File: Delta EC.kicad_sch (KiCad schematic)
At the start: 43 parts, among them J1 USB_C_Receptacle_USB2.0_16P, J2 SOICbite, J3 FFC Daughter side, J4 FFC Main side, J5 JSB USB, U1 STM32G474CBTx, U2 USBLC6-2SC6, U3 TPS7A2033, Y1 8Mhz 12pF

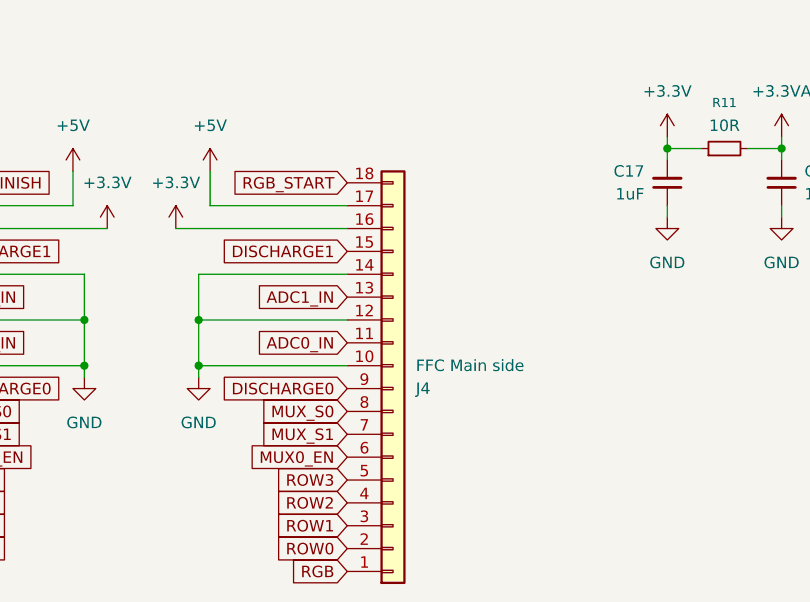
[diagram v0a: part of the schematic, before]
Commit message: 17.04.2026
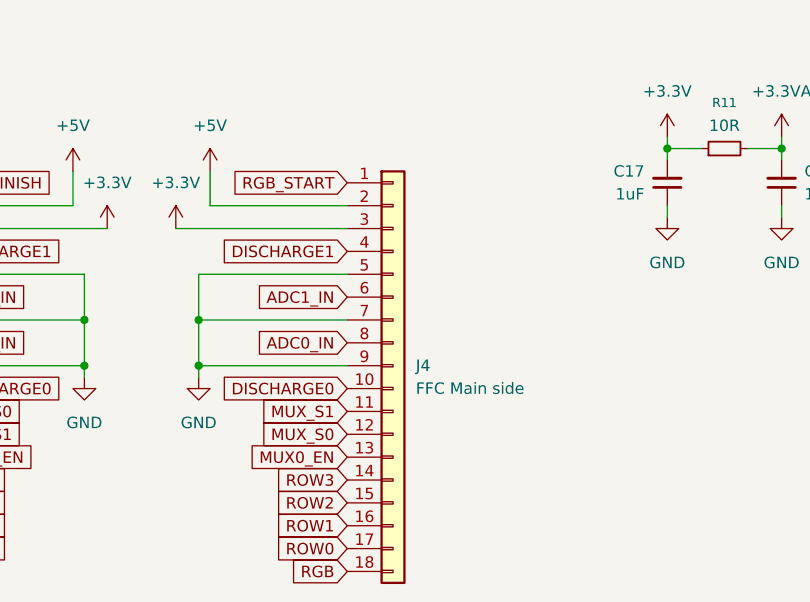
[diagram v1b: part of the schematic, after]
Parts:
- J3, J4: footprint Connector_FFC-FPC:JUSHUO_AFA07-S18FCA-00_1x18-1MP_P1.0mm_Horizontal -> Connector_FFC-FPC:Amphenol_F32Q-1A7x1-11018_1x18-1MP_P0.5mm_Horizontal
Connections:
- net +3.3V: now also J4.3 (Pin_3); no longer J4.16 (Pin_16)
- net +5V: now also J4.2 (Pin_2); no longer J4.17 (Pin_17)
- net ADC0_IN: now also J4.8 (Pin_8); no longer J4.11 (Pin_11)
- net ADC1_IN: now also J4.6 (Pin_6); no longer J4.13 (Pin_13)
- net DISCHARGE0: now also J4.10 (Pin_10); no longer J4.9 (Pin_9)
- net DISCHARGE1: now also J4.4 (Pin_4); no longer J4.15 (Pin_15)
- net GND: now also J4.5 (Pin_5), J4.7 (Pin_7), J4.9 (Pin_9); no longer J4.10 (Pin_10), J4.12 (Pin_12), J4.14 (Pin_14)
- net MUX0_EN: now also J4.13 (Pin_13); no longer J4.6 (Pin_6)
- net MUX_S0: now also J4.12 (Pin_12); no longer J4.8 (Pin_8)
- net MUX_S1: now also J4.11 (Pin_11); no longer J4.7 (Pin_7)
- net RGB: now also J4.18 (Pin_18); no longer J4.1 (Pin_1)
- net RGB_START: now also J4.1 (Pin_1); no longer J4.18 (Pin_18)
- net ROW0: now also J4.17 (Pin_17); no longer J4.2 (Pin_2)
- net ROW1: now also J4.16 (Pin_16); no longer J4.3 (Pin_3)
- net ROW2: now also J4.15 (Pin_15); no longer J4.4 (Pin_4)
- net ROW3: now also J4.14 (Pin_14); no longer J4.5 (Pin_5)
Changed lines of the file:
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@@
 	(global_label "MUX_S1"
 		(shape input)
-		(at 157.48 180.34 180)
+		(at 157.48 177.8 180)
 		(fields_autoplaced yes)
 		(effects
@@
 		)
 		(property "Intersheetrefs" "${INTERSHEET_REFS}"
-			(at 147.1168 180.34 0)
+			(at 147.1168 177.8 0)
 			(effects
 				(font
@@
 	(global_label "MUX_S0"
 		(shape input)
-		(at 157.48 177.8 180)
+		(at 157.48 180.34 180)
 		(fields_autoplaced yes)
 		(effects
@@
 		)
 		(property "Intersheetrefs" "${INTERSHEET_REFS}"
-			(at 147.1168 177.8 0)
+			(at 147.1168 180.34 0)
 			(effects
 				(font
@@
 			)
 		)
-		(property "Footprint" "Connector_FFC-FPC:JUSHUO_AFA07-S18FCA-00_1x18-1MP_P1.0mm_Horizontal"
+		(property "Footprint" "Connector_FFC-FPC:Amphenol_F32Q-1A7x1-11018_1x18-1MP_P0.5mm_Horizontal"
 			(at 106.68 172.72 0)
 			(effects
@@
 	(symbol
 		(lib_id "Connector_Generic:Conn_01x18")
-		(at 162.56 175.26 0)
-		(mirror x)
+		(at 162.56 172.72 0)
 		(unit 1)
 		(exclude_from_sim no)
@@
 		(dnp no)
 		(property "Reference" "J4"
-			(at 165.1 175.2601 0)
+			(at 165.1 172.7199 0)
 			(effects
 				(font
@@
 		)
 		(property "Value" "FFC Main side"
-			(at 165.1 172.7201 0)
+			(at 165.1 175.2599 0)
 			(effects
 				(font
@@
 			)
 		)
-		(property "Footprint" "Connector_FFC-FPC:JUSHUO_AFA07-S18FCA-00_1x18-1MP_P1.0mm_Horizontal"
-			(at 162.56 175.26 0)
+		(property "Footprint" "Connector_FFC-FPC:Amphenol_F32Q-1A7x1-11018_1x18-1MP_P0.5mm_Horizontal"
+			(at 162.56 172.72 0)
 			(effects
 				(font
@@
 		)
 		(property "Datasheet" "~"
-			(at 162.56 175.26 0)
+			(at 162.56 172.72 0)
 			(effects
 				(font
@@
 		)
 		(property "Description" "Generic connector, single row, 01x18, script generated (kicad-library-utils/schlib/autogen/connector/)"
-			(at 162.56 175.26 0)
+			(at 162.56 172.72 0)
 			(effects
 				(font
